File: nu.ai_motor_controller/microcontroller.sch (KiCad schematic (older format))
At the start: 4 parts

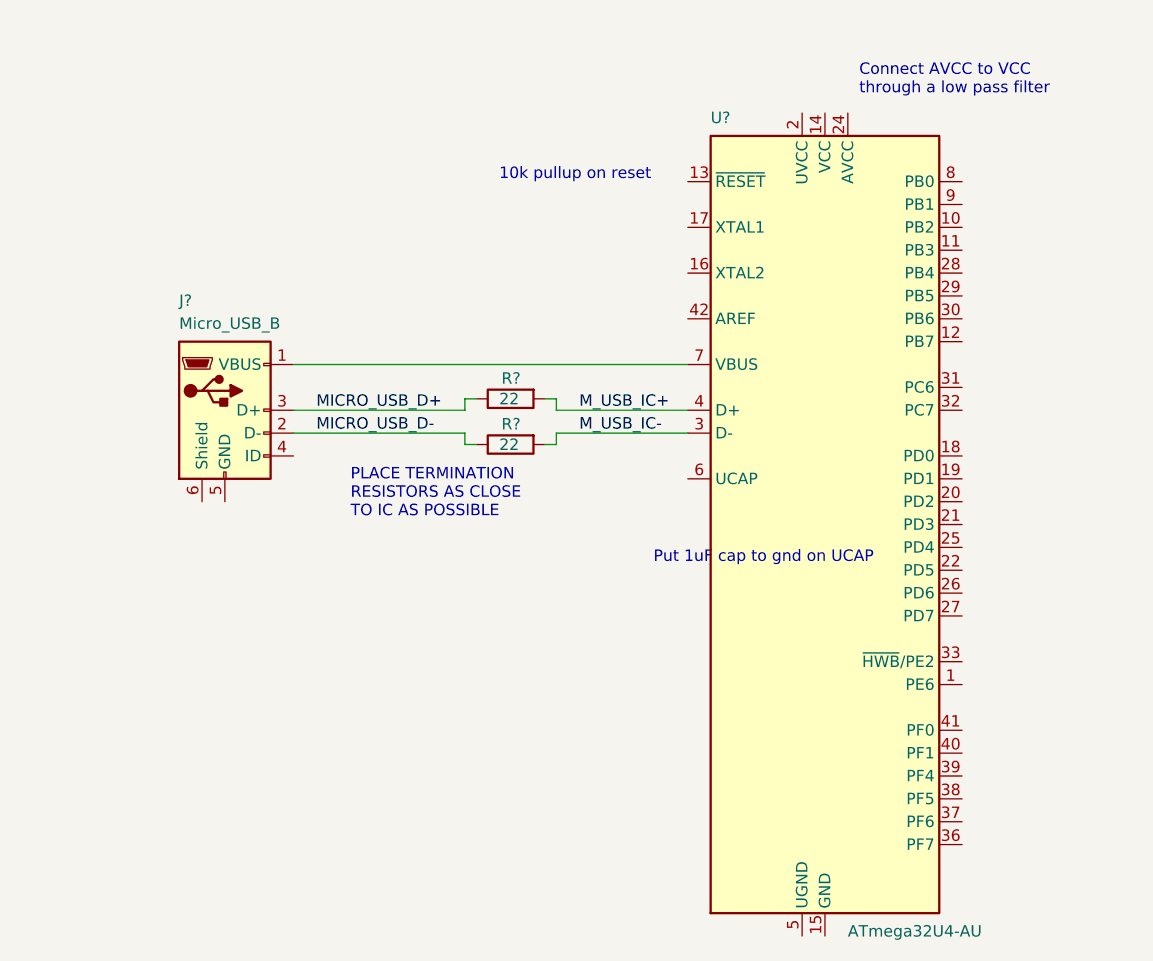
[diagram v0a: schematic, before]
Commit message: automated commit
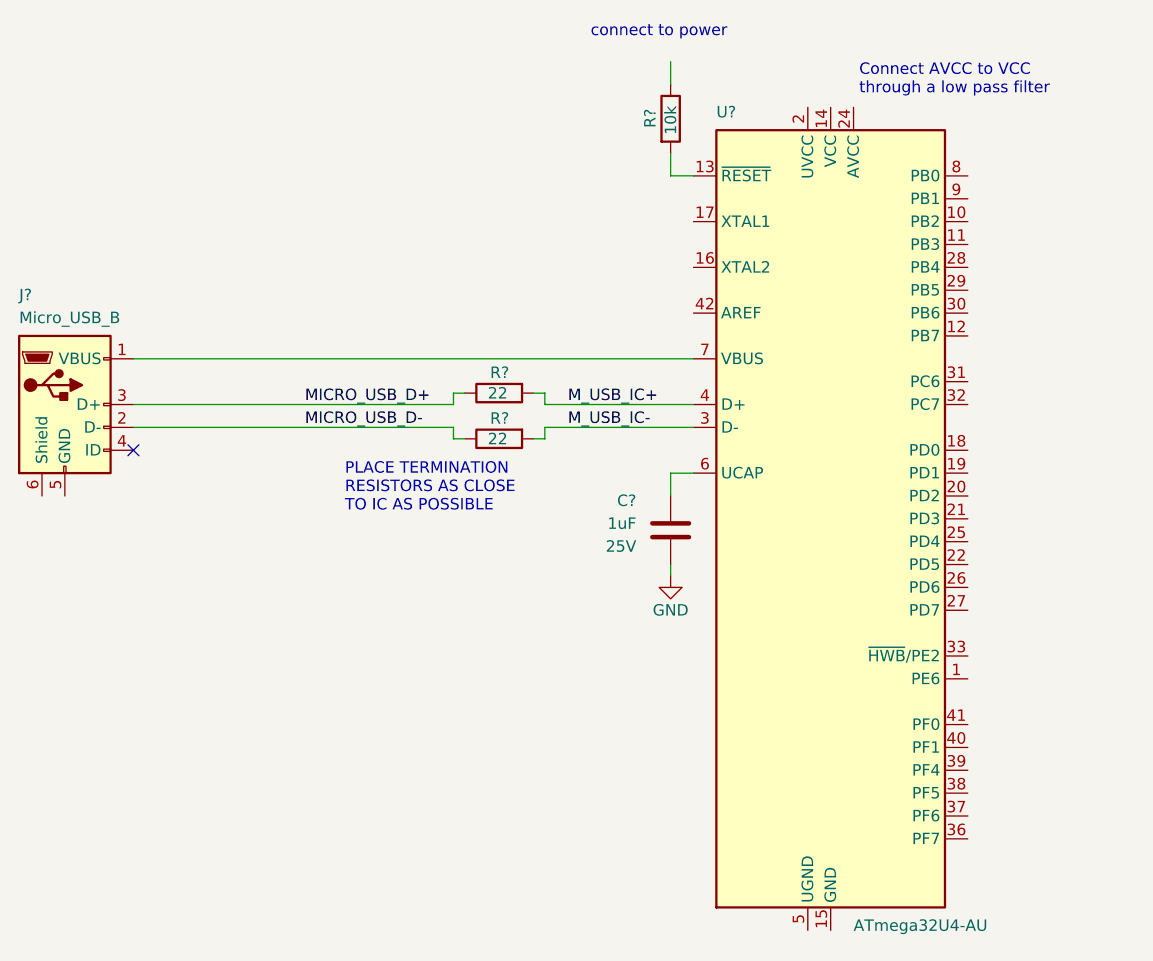
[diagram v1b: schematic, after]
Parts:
- added C?: CL10B105KA8NNNC, Capacitor_SMD:C_0603_1608Metric, symbol custom:CL10B105KA8NNNC
- added R?: CR0603-JW-103ELF, 0603, symbol custom:CR0603-JW-103ELF
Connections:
- net labels added: GND
- wire segments 13 -> 19
- no-connect marks 0 -> 1
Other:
- note added: "connect to power\n"
- note removed: "10k pullup on reset"
- note removed: "Put 1uF cap to gnd on UCAP"
- moved on the sheet: J?, R?, U?
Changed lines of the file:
@@
 L MCU_Microchip_ATmega:ATmega32U4-AU U?
 U 1 1 5C3ED06E
-P 5325 3725
-F 0 "U?" H 4825 5475 50  0000 L BNN
-F 1 "ATmega32U4-AU" H 5425 1975 50  0000 L TNN
-F 2 "Package_QFP:TQFP-44_10x10mm_P0.8mm" H 5325 3725 50  0001 C CIN
-F 3 "http://ww1.microchip.com/downloads/en/DeviceDoc/Atmel-7766-8-bit-AVR-ATmega16U4-32U4_Datasheet.pdf" H 5325 3725 50  0001 C CNN
-	1    5325 3725
+P 5350 3700
+F 0 "U?" H 4850 5450 50  0000 L BNN
+F 1 "ATmega32U4-AU" H 5450 1950 50  0000 L TNN
+F 2 "Package_QFP:TQFP-44_10x10mm_P0.8mm" H 5350 3700 50  0001 C CIN
+F 3 "http://ww1.microchip.com/downloads/en/DeviceDoc/Atmel-7766-8-bit-AVR-ATmega16U4-32U4_Datasheet.pdf" H 5350 3700 50  0001 C CNN
+	1    5350 3700
 	1    0    0    -1
 $EndComp
@@
 L custom:DX4R105JJCR1800 J?
 U 1 1 5C3ED2E2
-P 2700 3225
-F 0 "J?" H 2500 3675 50  0000 L BNN
-F 1 "DX4R105JJCR1800" H 2400 2425 50  0001 L BNN
-F 2 "" H 2850 3175 50  0001 C CNN
-F 3 "SJ113218.pdf" H 2850 3175 50  0001 L BNN
-F 4 "Micro_USB_B" H 2500 3575 50  0000 L BNN "Description"
-	1    2700 3225
+P 2000 3200
+F 0 "J?" H 1800 3650 50  0000 L BNN
+F 1 "DX4R105JJCR1800" H 1700 2400 50  0001 L BNN
+F 2 "" H 2150 3150 50  0001 C CNN
+F 3 "SJ113218.pdf" H 2150 3150 50  0001 L BNN
+F 4 "Micro_USB_B" H 1800 3550 50  0000 L BNN "Description"
+	1    2000 3200
 	1    0    0    -1
 $EndComp
-Text Label 3100 3225 0    50   ~ 0
+Text Label 3050 3200 0    50   ~ 0
 MICRO_USB_D+
-Text Label 3100 3325 0    50   ~ 0
+Text Label 3050 3300 0    50   ~ 0
 MICRO_USB_D-
-Text Notes 3250 3700 0    50   ~ 0
+Text Notes 3225 3675 0    50   ~ 0
 PLACE TERMINATION\nRESISTORS AS CLOSE\nTO IC AS POSSIBLE
 Wire Wire Line
-	3000 3025 4725 3025
-Text Notes 4575 3900 0    50   ~ 0
-Put 1uF cap to gnd on UCAP
-Text Notes 3900 2225 0    50   ~ 0
-10k pullup on reset
+	2300 3000 4750 3000
 Text Notes 5475 1850 0    50   ~ 0
 Connect AVCC to VCC\nthrough a low pass filter
@@
 L custom:RMCF0603FT22R0 R?
 U 1 1 5C4048F8
-P 3950 3375
-F 0 "R?" V 3890 3335 50  0000 L BNN
-F 1 "RMCF0603FT22R0" V 4075 3050 50  0001 L BNN
-F 2 "0603" V 4150 3275 50  0001 L BNN
-F 3 "~/datasheets/SEI-RMCF_RMCP.pdf" V 4250 3425 50  0001 C CNN
-F 4 "22" V 3980 3325 50  0000 L BNN "Resistance"
-	1    3950 3375
+P 3900 3350
+F 0 "R?" V 3840 3310 50  0000 L BNN
+F 1 "RMCF0603FT22R0" V 4025 3025 50  0001 L BNN
+F 2 "0603" V 4100 3250 50  0001 L BNN
+F 3 "~/datasheets/SEI-RMCF_RMCP.pdf" V 4200 3400 50  0001 C CNN
+F 4 "22" V 3930 3300 50  0000 L BNN "Resistance"
+	1    3900 3350
 	0    1    1    0
 $EndComp
@@
 L custom:RMCF0603FT22R0 R?
 U 1 1 5C404A44
-P 3950 3175
-F 0 "R?" V 3890 3135 50  0000 L BNN
-F 1 "RMCF0603FT22R0" V 4075 2850 50  0001 L BNN
-F 2 "0603" V 4150 3075 50  0001 L BNN
-F 3 "~/datasheets/SEI-RMCF_RMCP.pdf" V 4250 3225 50  0001 C CNN
-F 4 "22" V 3980 3125 50  0000 L BNN "Resistance"
-	1    3950 3175
+P 3900 3150
+F 0 "R?" V 3840 3110 50  0000 L BNN
+F 1 "RMCF0603FT22R0" V 4025 2825 50  0001 L BNN
+F 2 "0603" V 4100 3050 50  0001 L BNN
+F 3 "~/datasheets/SEI-RMCF_RMCP.pdf" V 4200 3200 50  0001 C CNN
+F 4 "22" V 3930 3100 50  0000 L BNN "Resistance"
+	1    3900 3150
 	0    1    1    0
 $EndComp
 Wire Wire Line
-	4100 3175 4150 3175
+	4050 3150 4100 3150
 Wire Wire Line
-	4150 3175 4150 3225
+	4100 3150 4100 3200
 Wire Wire Line
-	4150 3225 4725 3225
+	4100 3300 4100 3350
 Wire Wire Line
-	4725 3325 4150 3325
+	4100 3350 4050 3350
 Wire Wire Line
-	4150 3325 4150 3375
+	3750 3350 3700 3350
 Wire Wire Line
-	4150 3375 4100 3375
+	3700 3300 2300 3300
 Wire Wire Line
-	3800 3375 3750 3375
+	3700 3300 3700 3350
 Wire Wire Line
-	3750 3325 3000 3325
+	2300 3200 3700 3200
 Wire Wire Line
-	3750 3325 3750 3375
+	3700 3200 3700 3150
 Wire Wire Line
-	3000 3225 3750 3225
+	3700 3150 3750 3150
+Text Label 4200 3200 0    50   ~ 0
+M_USB_IC+
+Text Label 4200 3300 0    50   ~ 0
+M_USB_IC-
+$Comp
+L custom:CL10B105KA8NNNC C?
+U 1 1 5C414E9B
+P 4650 3750
+F 0 "C?" H 4800 3850 50  0000 L BNN
+F 1 "CL10B105KA8NNNC" H 3700 3300 50  0001 L BNN
+F 2 "Capacitor_SMD:C_0603_1608Metric" H 3700 3200 50  0001 L BNN
+F 3 "datasheets/CL10B105KA8NNNC.pdf" H 3700 3100 50  0001 L BNN
+F 4 "1uF" H 4800 3750 50  0000 L BNN "Capacitance"
+F 5 "25V" H 4800 3650 50  0000 L BNN "Rating"
+	1    4650 3750
+	-1   0    0    -1
+$EndComp
+$Comp
+L power:GND #PWR?
+U 1 1 5C414F68
+P 4650 3950
+F 0 "#PWR?" H 4650 3700 50  0001 C CNN
+F 1 "GND" H 4650 3800 50  0000 C CNN
+F 2 "" H 4650 3950 50  0001 C CNN
+F 3 "" H 4650 3950 50  0001 C CNN
+	1    4650 3950
+	1    0    0    -1
+$EndComp
 Wire Wire Line
-	3750 3225 3750 3175
+	4650 3950 4650 3900
 Wire Wire Line
-	3750 3175 3800 3175
-Text Label 4250 3225 0    50   ~ 0
-M_USB_IC+
-Text Label 4250 3325 0    50   ~ 0
-M_USB_IC-
+	4650 3600 4650 3500
+Wire Wire Line
+	4650 3500 4750 3500
+Wire Wire Line
+	4100 3300 4750 3300
+Wire Wire Line
+	4100 3200 4750 3200
+$Comp
+L custom:CR0603-JW-103ELF R?
+U 1 1 5C41A4AA
+P 4650 1950
+F 0 "R?" V 4590 1910 50  0000 L BNN
+F 1 "CR0603-JW-103ELF" V 4775 1625 50  0001 L BNN
+F 2 "0603" V 4850 1850 50  0001 L BNN
+F 3 "~/datasheets/chpreztr.pdf" V 4950 1500 50  0001 L BNN
+F 4 "10k" V 4680 1880 50  0000 L BNN "Resistance"
+	1    4650 1950
+	1    0    0    -1
+$EndComp
+Wire Wire Line
+	4650 2100 4650 2200
+Wire Wire Line
+	4650 2200 4750 2200
+Wire Wire Line
+	4650 1800 4650 1700
+Text Notes 4300 1600 0    50   ~ 0
+connect to power\n
+NoConn ~ 2300 3400
 $EndSCHEMATC
